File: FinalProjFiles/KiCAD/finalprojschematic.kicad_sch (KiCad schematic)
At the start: 9 parts, among them M1 Motor_Servo, M2 Motor_Servo, M3 Motor_Servo

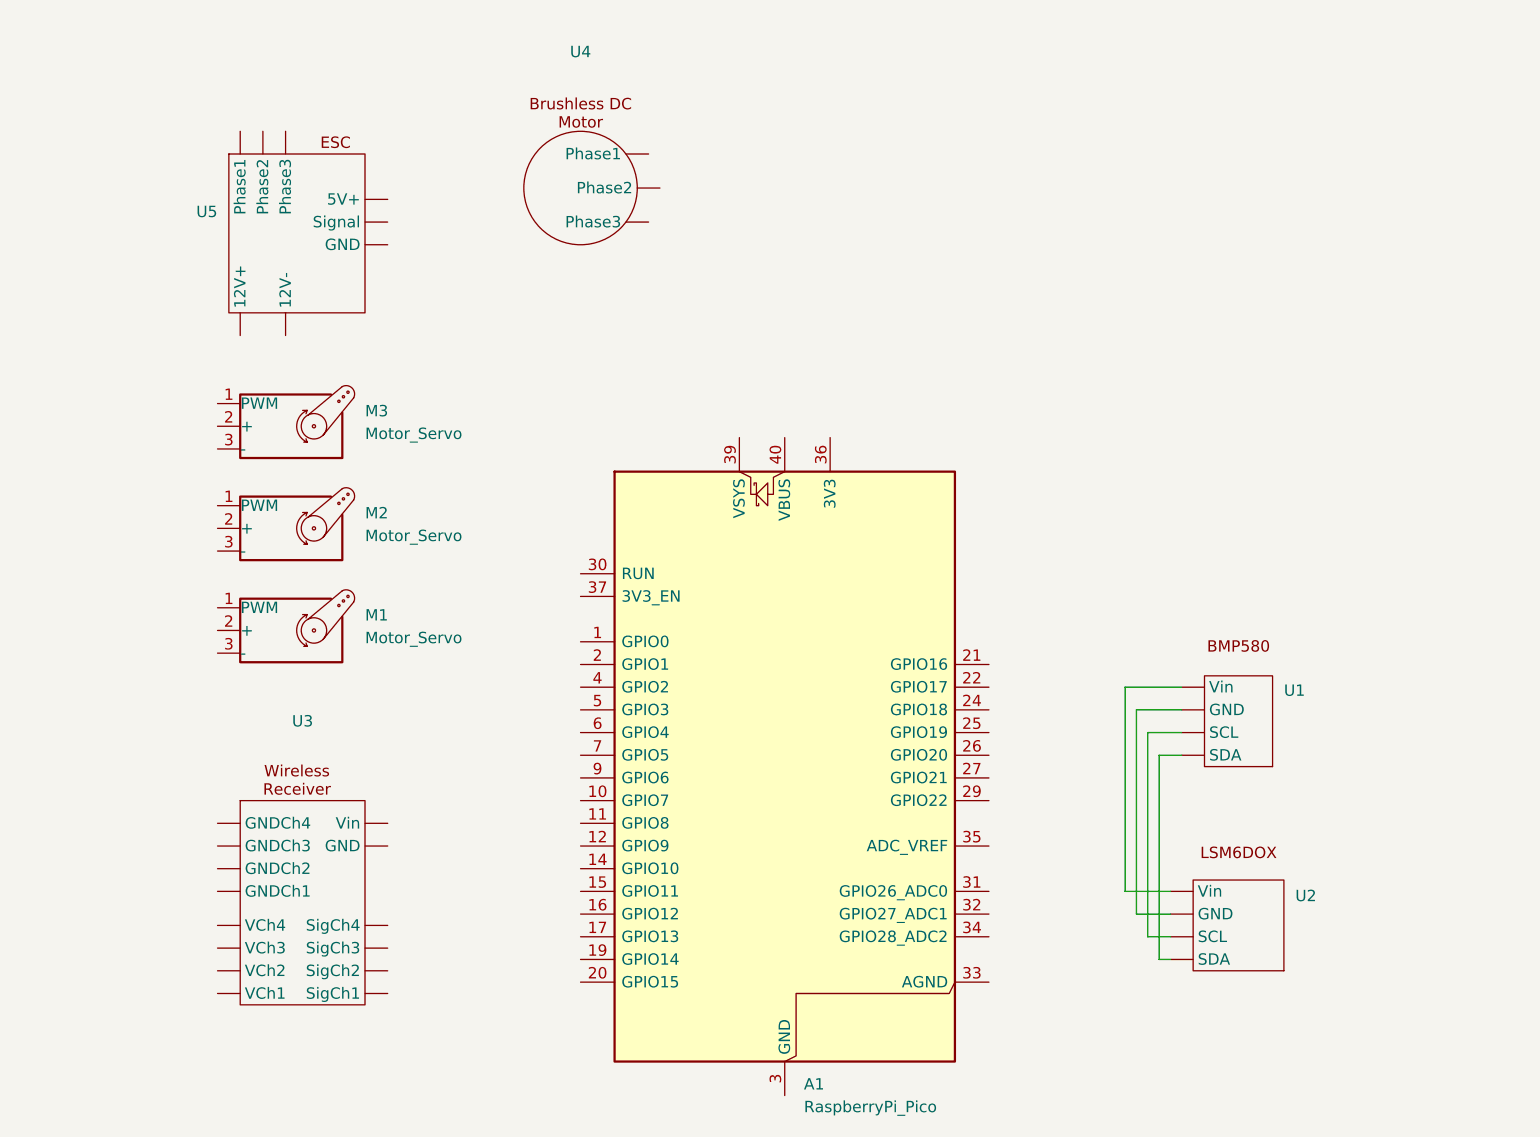
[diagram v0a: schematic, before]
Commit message: Finished Schematic
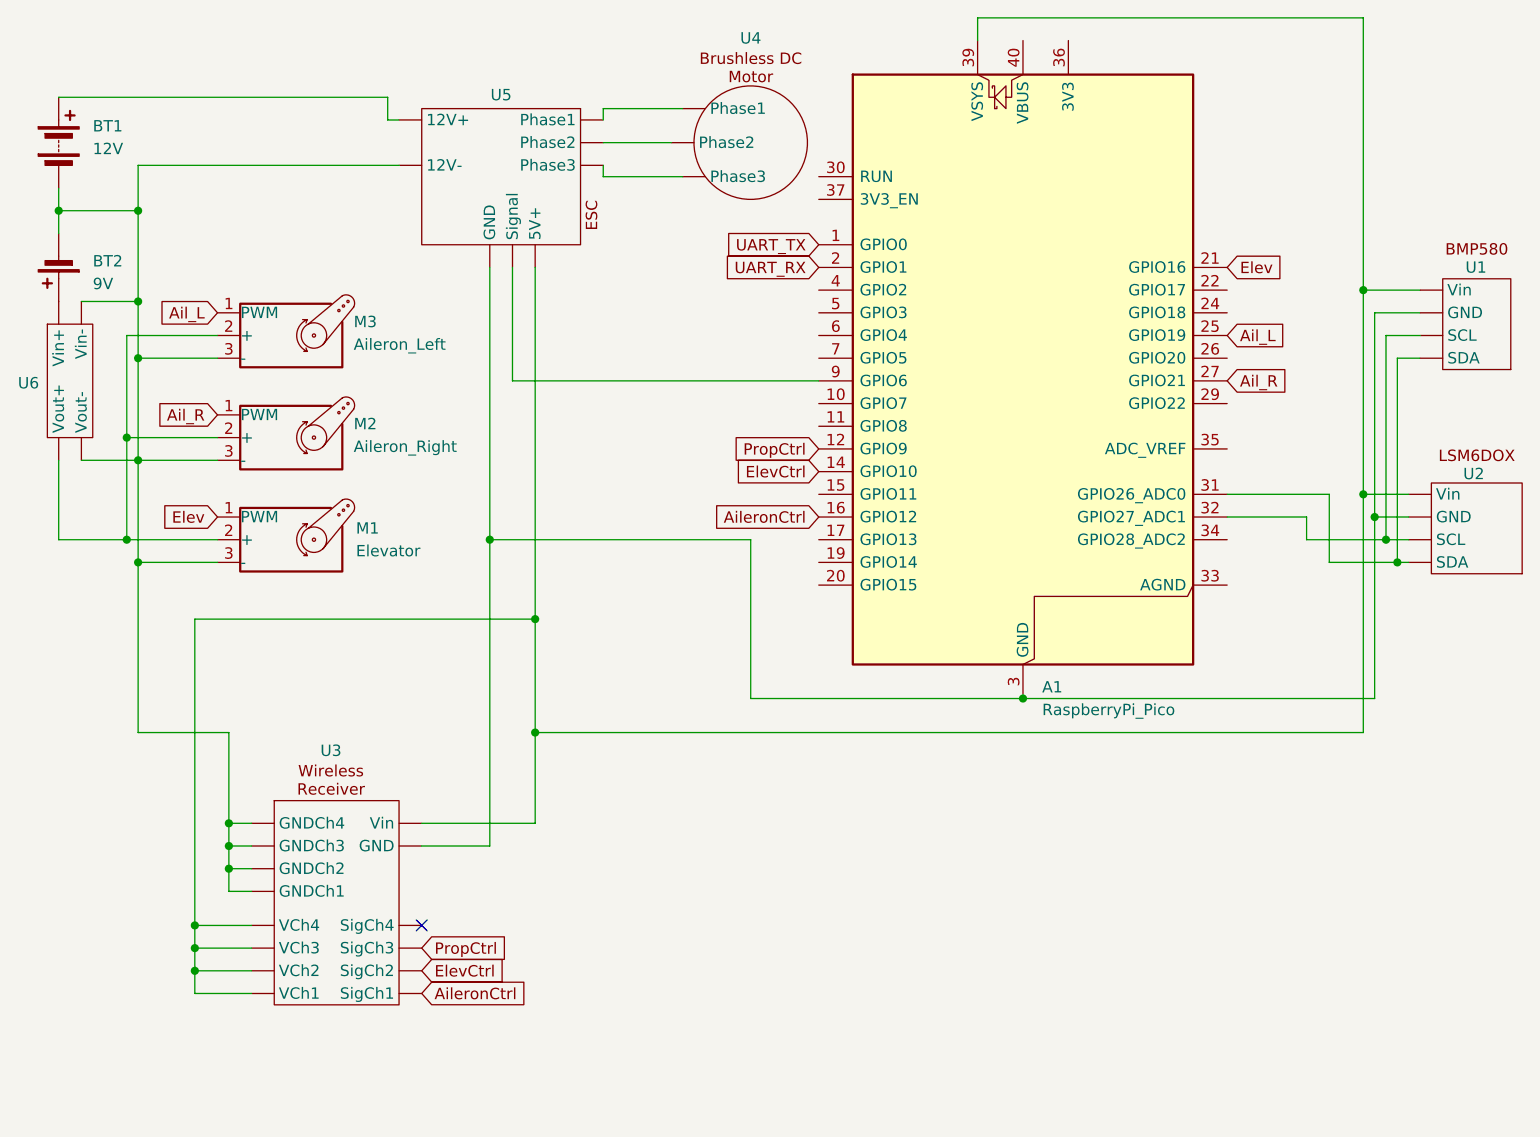
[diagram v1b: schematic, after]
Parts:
- added BT1: 12V, symbol Device:Battery
- added BT2: 9V, symbol Device:Battery_Cell
- added U6: ~, symbol projectLibrary:5V_Regulator
- M1: value Motor_Servo -> Elevator
- M2: value Motor_Servo -> Aileron_Right
- M3: value Motor_Servo -> Aileron_Left
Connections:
- net at U1. (Vin), U2. (Vin): now also A1.39 (VSYS), U3. (SigCh1), U5. (GND)
- net UART_TX: now reaches A1.1 (GPIO0)
- net PropCtrl: now reaches A1.12 (GPIO9)
- net PropCtrl: now also U3. (SigCh1)
- net at A1.13 (GND), A1.18 (GND), A1.23 (GND)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: now also U1. (Vin), U2. (Vin), U3. (SigCh1), U5. (GND)
- net ElevCtrl: now reaches A1.14 (GPIO10)
- net ElevCtrl: now also U3. (SigCh1)
- net AileronCtrl: now reaches A1.16 (GPIO12)
- net AileronCtrl: now also U3. (SigCh1)
- net UART_RX: now reaches A1.2 (GPIO1)
- net Elev: now reaches A1.21 (GPIO16)
- net Elev: now also M1.1 (PWM)
- net Ail_L: now reaches A1.25 (GPIO19)
- net Ail_L: now also M3.1 (PWM)
- net Ail_R: now reaches A1.27 (GPIO21)
- net Ail_R: now also M2.1 (PWM)
- net at A1.31 (GPIO26_ADC0): now also U1. (Vin), U2. (Vin)
- net at A1.32 (GPIO27_ADC1): now also U1. (Vin), U2. (Vin)
- net at A1.9 (GPIO6): now also U5. (GND)
- net at M1.2 (+): now also M2.2 (+), M3.2 (+), U6. (Vout-)
- net at M1.3 (-): now also M2.3 (-), M3.3 (-), U3. (SigCh1), U5. (GND), BT1.2 (-), BT2.2 (-), U6. (Vout-)
- net at U4. (Phase2): now also U5. (GND)
- net at U5. (GND): now also BT1.1 (+)
- new net: BT2.1 (+), U6. (Vout-)
- new net: U4. (Phase2), U5. (GND) (x2)
- no-connect marks 0 -> 1
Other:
- company: (none) -> ECE414
- title: (none) -> Final Project Schematic
- moved on the sheet: A1, M1, M2, M3, U1, U2, U3, U4, U5
